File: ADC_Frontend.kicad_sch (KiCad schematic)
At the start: 23 parts, among them U701 THS4551xRGT

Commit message: (sch) fix THS4551 3D model
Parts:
- U701: footprint Package_DFN_QFN:VQFN-16-1EP_3x3mm_P0.5mm_EP1.68x1.68mm_ThermalVias -> grootvoet:VQFN-16-1EP_3x3mm_P0.5mm_EP1.68x1.68mm_ThermalVias
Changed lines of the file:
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@@
       (effects (font (size 1.27 1.27)) (justify left))
     )
-    (property "Footprint" "Package_DFN_QFN:VQFN-16-1EP_3x3mm_P0.5mm_EP1.68x1.68mm_ThermalVias" (at 134.62 119.38 0)
+    (property "Footprint" "grootvoet:VQFN-16-1EP_3x3mm_P0.5mm_EP1.68x1.68mm_ThermalVias" (at 134.62 119.38 0)
       (effects (font (size 1.27 1.27)) hide)
     )
@@
       (effects (font (size 1.27 1.27)) (justify left))
     )
-    (property "Footprint" "Package_DFN_QFN:VQFN-16-1EP_3x3mm_P0.5mm_EP1.68x1.68mm_ThermalVias" (at 163.195 55.245 0)
-      (effects (font (size 1.27 1.27)) hide)
-    )
+    (property "Footprint" "grootvoet:VQFN-16-1EP_3x3mm_P0.5mm_EP1.68x1.68mm_ThermalVias" (at 163.195 55.245 0)
+      (effects (font (size 1.27 1.27)) hide)
+    )

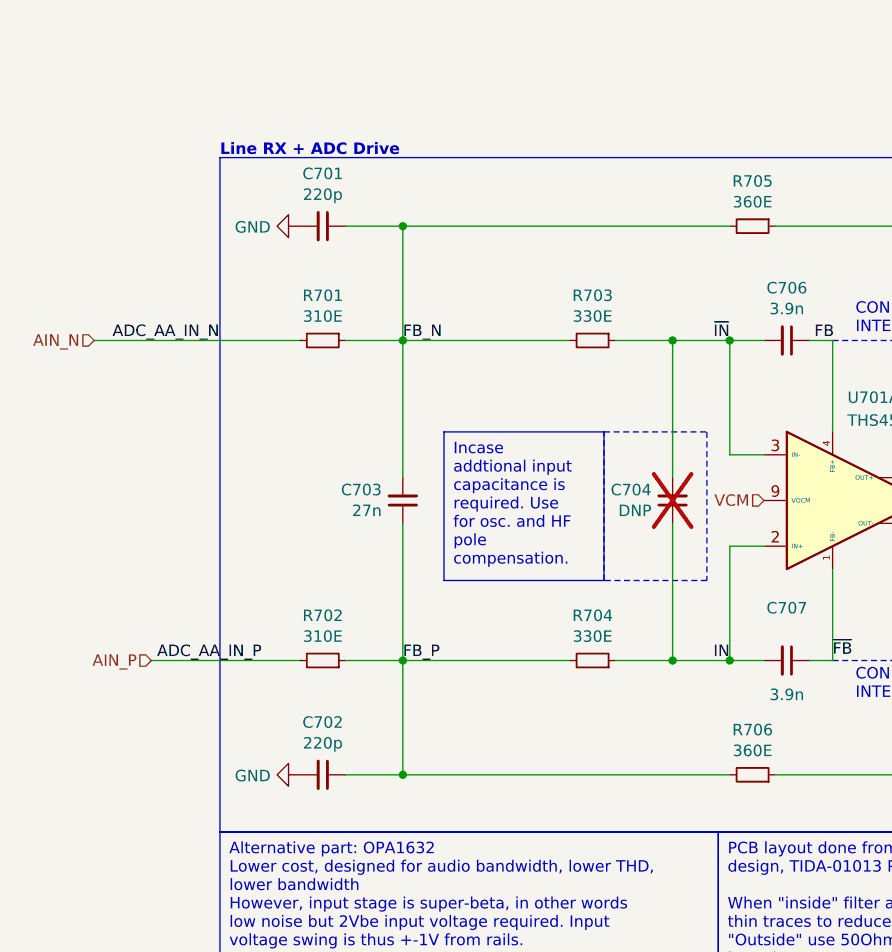
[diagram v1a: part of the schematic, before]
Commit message: (sch) run DRC
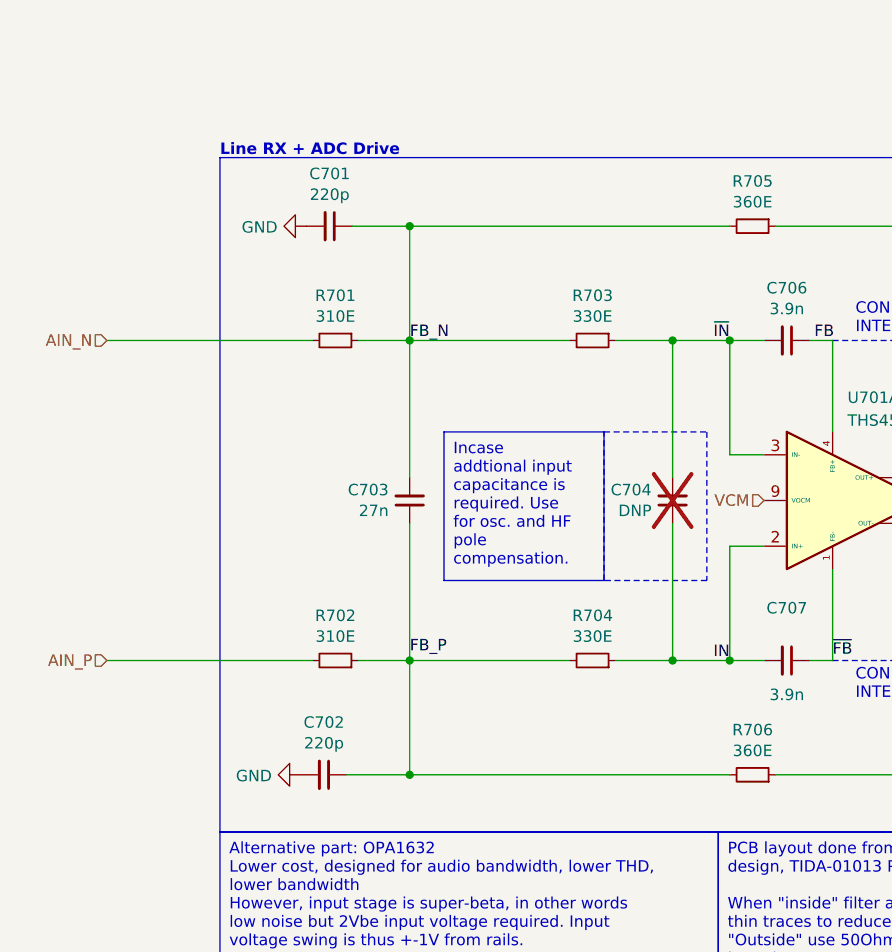
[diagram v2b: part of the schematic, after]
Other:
- moved on the sheet: C701, C703, R701, R702
